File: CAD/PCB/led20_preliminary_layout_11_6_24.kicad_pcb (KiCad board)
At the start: 2 copper layers, 55 x 55 mm, 33 parts, among them U3 Battery, U6 JST

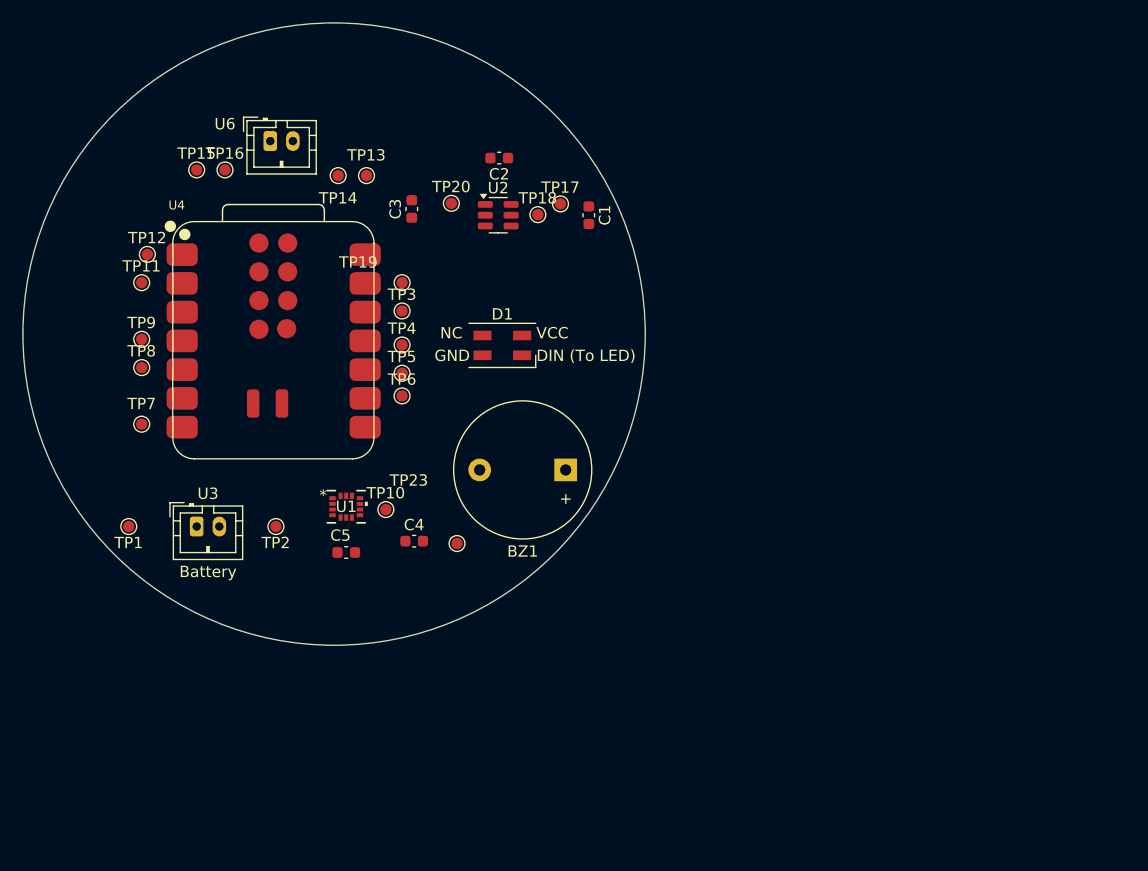
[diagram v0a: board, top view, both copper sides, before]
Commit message: Resubmit
see previous notes
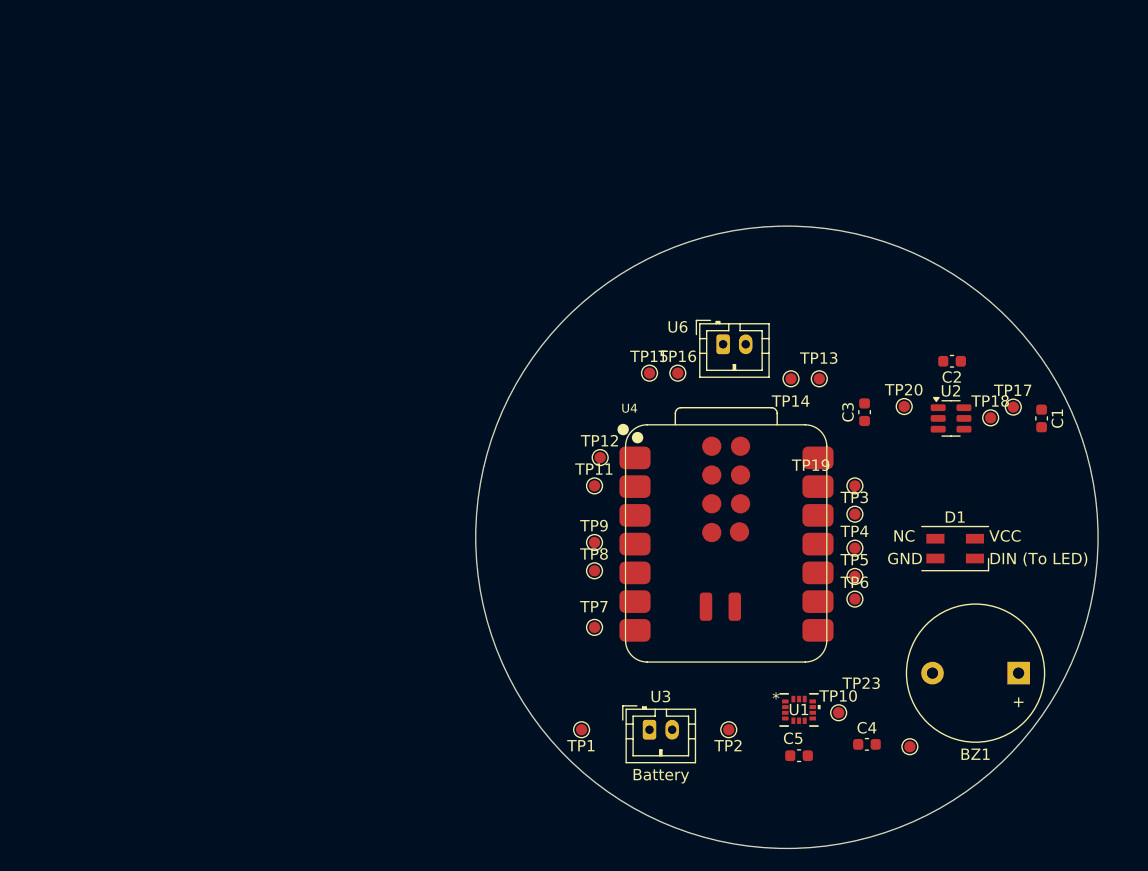
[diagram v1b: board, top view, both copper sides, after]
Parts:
- moved BZ1 43.8 mm to (163.6, 90.0)
- moved C2 43.8 mm to (157.7, 62.5)
- moved C3 43.8 mm to (150.0, 67.0)
- moved D1 43.8 mm to (158.0, 79.0)
- moved TP1 43.8 mm to (125.0, 95.0)
- moved TP11 43.8 mm to (126.1, 73.5)
- moved TP12 43.8 mm to (126.6, 71.0)
- moved TP13 43.8 mm to (146.0, 64.0)
- moved TP14 43.8 mm to (143.5, 64.0)
- moved TP15 43.8 mm to (131.0, 63.5)
- moved TP16 43.8 mm to (133.5, 63.5)
- moved TP2 43.8 mm to (138.0, 95.0)
- moved TP20 43.8 mm to (153.5, 66.5)
- moved TP23 43.8 mm to (154.0, 96.5)
- moved TP7 43.8 mm to (126.1, 86.0)
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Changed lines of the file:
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@@
 		(legacy_teardrops no)
 	)
-	(paper "A5")
+	(paper "A4")
 	(title_block
 		(title "LED20 Preliminary PCB Layout")
@@
 		(allow_soldermask_bridges_in_footprints no)
 		(pcbplotparams
-			(layerselection 0x0001000_7ffffffe)
+			(layerselection 0x0040000_7ffffffe)
 			(plot_on_all_layers_selection 0x7ffffff_80000001)
 			(disableapertmacros no)
@@
 			(drillshape 0)
 			(scaleselection 1)
-			(outputdirectory "./")
+			(outputdirectory "")
 		)
 	)
@@
 	(footprint "Connector_JST:JST_PH_B2B-PH-K_1x02_P2.00mm_Vertical"
 		(layer "F.Cu")
-		(at 97.5 43)
+		(at 137.5 60.95)
 		(descr "JST PH series connector, B2B-PH-K (http://www.jst-mfg.com/product/pdf/eng/ePH.pdf), generated with kicad-footprint-generator")
 		(tags "connector JST PH side entry")
@@
 	(footprint "TestPoint:TestPoint_Pad_D1.0mm"
 		(layer "F.Cu")
-		(at 98 77.05 180)
+		(at 138 95 180)
 		(descr "SMD pad as test Point, diameter 1.0mm")
 		(tags "test point SMD pad")
@@
 	(footprint "Led20:ChargePump"
 		(layer "F.Cu")
-		(at 117.6375 49.55)
+		(at 157.6375 67.5)
 		(descr "SOT, 6 Pin (~), generated with kicad-footprint-generator ipc_gullwing_generator.py")
 		(tags "SOT TO_SOT_SMD")
@@
 	(footprint "TestPoint:TestPoint_Pad_D1.0mm"
 		(layer "F.Cu")
-		(at 107.7103 75.549999)
+		(at 147.7103 93.499999)
 		(descr "SMD pad as test Point, diameter 1.0mm")
 		(tags "test point SMD pad")
@@
 	(footprint "TestPoint:TestPoint_Pad_D1.0mm"
 		(layer "F.Cu")
-		(at 114 78.55)
+		(at 154 96.5)
 		(descr "SMD pad as test Point, diameter 1.0mm")
 		(tags "test point SMD pad")
@@
 	(footprint "LED_SMD:LED_SK6812MINI_PLCC4_3.5x3.5mm_P1.75mm"
 		(layer "F.Cu")
-		(at 118 61.05)
+		(at 158 79)
 		(descr "3.5mm x 3.5mm PLCC4 Addressable RGB LED NeoPixel, https://cdn-shop.adafruit.com/product-files/2686/SK6812MINI_REV.01-1-2.pdf")
 		(tags "LED RGB NeoPixel Mini PLCC-4 3535")
@@
 	(footprint "Capacitor_SMD:C_0603_1608Metric"
 		(layer "F.Cu")
-		(at 110 49 90)
+		(at 150 66.95 90)
 		(descr "Capacitor SMD 0603 (1608 Metric), square (rectangular) end terminal, IPC_7351 nominal, (Body size source: IPC-SM-782 page 76, https://www.pcb-3d.com/wordpress/wp-content/uploads/ipc-sm-782a_amendment_1_and_2.pdf), generated with kicad-footprint-generator")
 		(tags "capacitor")
@@
 	(footprint "TestPoint:TestPoint_Pad_D1.0mm"
 		(layer "F.Cu")
-		(at 86.1444 63.01)
+		(at 126.1444 80.96)
 		(descr "SMD pad as test Point, diameter 1.0mm")
 		(tags "test point SMD pad")
@@
 	(footprint "TestPoint:TestPoint_Pad_D1.0mm"
 		(layer "F.Cu")
-		(at 91 45.55)
+		(at 131 63.5)
 		(descr "SMD pad as test Point, diameter 1.0mm")
 		(tags "test point SMD pad")
@@
 	(footprint "Connector_JST:JST_PH_B2B-PH-K_1x02_P2.00mm_Vertical"
 		(layer "F.Cu")
-		(at 91 77.05)
+		(at 131 95)
 		(descr "JST PH series connector, B2B-PH-K (http://www.jst-mfg.com/product/pdf/eng/ePH.pdf), generated with kicad-footprint-generator")
 		(tags "connector JST PH side entry")
@@
 	(footprint "TestPoint:TestPoint_Pad_D1.0mm"
 		(layer "F.Cu")
-		(at 93.5 45.55)
+		(at 133.5 63.5)
 		(descr "SMD pad as test Point, diameter 1.0mm")
 		(tags "test point SMD pad")
@@
 	(footprint "Capacitor_SMD:C_0603_1608Metric"
 		(layer "F.Cu")
-		(at 104.2103 79.343699)
+		(at 144.2103 97.293699)
 		(descr "Capacitor SMD 0603 (1608 Metric), square (rectangular) end terminal, IPC_7351 nominal, (Body size source: IPC-SM-782 page 76, https://www.pcb-3d.com/wordpress/wp-content/uploads/ipc-sm-782a_amendment_1_and_2.pdf), generated with kicad-footprint-generator")
 		(tags "capacitor")
@@
 	(footprint "Led20:LGA-14L_2P5X3X0P83_STM-L"
 		(layer "F.Cu")
-		(at 104.2103 75.299999)
+		(at 144.2103 93.249999)
 		(tags "LSM6DSO32TR ")
 		(property "Reference" "U1"
@@
 	(footprint "TestPoint:TestPoint_Pad_D1.0mm"
 		(layer "F.Cu")
-		(at 86.1444 68.01)
+		(at 126.1444 85.96)
 		(descr "SMD pad as test Point, diameter 1.0mm")
 		(tags "test point SMD pad")
@@
 	(footprint "Led20:XIAO-ESP32-C6-SMD"
 		(layer "F.Cu")
-		(at 98 60.63)
+		(at 138 78.58)
 		(property "Reference" "U4"
 			(at -9.5 -11.5 0)
@@
 	(footprint "TestPoint:TestPoint_Pad_D1.0mm"
 		(layer "F.Cu")
-		(at 106 46.05)
+		(at 146 64)
 		(descr "SMD pad as test Point, diameter 1.0mm")
 		(tags "test point SMD pad")
@@
 	(footprint "TestPoint:TestPoint_Pad_D1.0mm"
 		(layer "F.Cu")
-		(at 121.1375 49.5)
+		(at 161.1375 67.45)
 		(descr "SMD pad as test Point, diameter 1.0mm")
 		(tags "test point SMD pad")
@@
 	(footprint "Capacitor_SMD:C_0603_1608Metric"
 		(layer "F.Cu")
-		(at 125.6375 49.55 -90)
+		(at 165.6375 67.5 -90)
 		(descr "Capacitor SMD 0603 (1608 Metric), square (rectangular) end terminal, IPC_7351 nominal, (Body size source: IPC-SM-782 page 76, https://www.pcb-3d.com/wordpress/wp-content/uploads/ipc-sm-782a_amendment_1_and_2.pdf), generated with kicad-footprint-generator")
 		(tags "capacitor")
@@
 	(footprint "Buzzer_Beeper:Buzzer_12x9.5RM7.6"
 		(layer "F.Cu")
-		(at 123.6 72.05 180)
+		(at 163.6 90 180)
 		(descr "Generic Buzzer, D12mm height 9.5mm with RM7.6mm")
 		(tags "buzzer")
@@
 	(footprint "TestPoint:TestPoint_Pad_D1.0mm"
 		(layer "F.Cu")
-		(at 103.5 46.05)
+		(at 143.5 64)
 		(descr "SMD pad as test Point, diameter 1.0mm")
 		(tags "test point SMD pad")
@@
 	(footprint "TestPoint:TestPoint_Pad_D1.0mm"
 		(layer "F.Cu")
-		(at 85 77.05 180)
+		(at 125 95 180)
 		(descr "SMD pad as test Point, diameter 1.0mm")
 		(tags "test point SMD pad")
@@
 	(footprint "Capacitor_SMD:C_0603_1608Metric"
 		(layer "F.Cu")
-		(at 117.725 44.5 180)
+		(at 157.725 62.45 180)
 		(descr "Capacitor SMD 0603 (1608 Metric), square (rectangular) end terminal, IPC_7351 nominal, (Body size source: IPC-SM-782 page 76, https://www.pcb-3d.com/wordpress/wp-content/uploads/ipc-sm-782a_amendment_1_and_2.pdf), generated with kicad-footprint-generator")
 		(tags "capacitor")
@@
 	(footprint "TestPoint:TestPoint_Pad_D1.0mm"
 		(layer "F.Cu")
-		(at 123.1375 48.55)
+		(at 163.1375 66.5)
 		(descr "SMD pad as test Point, diameter 1.0mm")
 		(tags "test point SMD pad")
@@
 	(footprint "TestPoint:TestPoint_Pad_D1.0mm"
 		(layer "F.Cu")
-		(at 109.1444 61.01)
+		(at 149.1444 78.96)
 		(descr "SMD pad as test Point, diameter 1.0mm")
 		(tags "test point SMD pad")
@@
 	(footprint "TestPoint:TestPoint_Pad_D1.0mm"
 		(layer "F.Cu")
-		(at 113.5 48.5)
+		(at 153.5 66.45)
 		(descr "SMD pad as test Point, diameter 1.0mm")
 		(tags "test point SMD pad")
@@
 	(footprint "TestPoint:TestPoint_Pad_D1.0mm"
 		(layer "F.Cu")
-		(at 109.1444 58.01)
+		(at 149.1444 75.96)
 		(descr "SMD pad as test Point, diameter 1.0mm")
 		(tags "test point SMD pad")
@@
 	(footprint "TestPoint:TestPoint_Pad_D1.0mm"
 		(layer "F.Cu")
-		(at 109.1444 55.51)
+		(at 149.1444 73.46)
 		(descr "SMD pad as test Point, diameter 1.0mm")
 		(tags "test point SMD pad")
@@
 	(footprint "TestPoint:TestPoint_Pad_D1.0mm"
 		(layer "F.Cu")
-		(at 109.1444 65.51)
+		(at 149.1444 83.46)
 		(descr "SMD pad as test Point, diameter 1.0mm")
 		(tags "test point SMD pad")
@@
 	(footprint "TestPoint:TestPoint_Pad_D1.0mm"
 		(layer "F.Cu")
-		(at 86.6444 53.01)
+		(at 126.6444 70.96)
 		(descr "SMD pad as test Point, diameter 1.0mm")
 		(tags "test point SMD pad")
@@
 	(footprint "TestPoint:TestPoint_Pad_D1.0mm"
 		(layer "F.Cu")
-		(at 86.1444 55.51)
+		(at 126.1444 73.46)
 		(descr "SMD pad as test Point, diameter 1.0mm")
 		(tags "test point SMD pad")
@@
 	(footprint "TestPoint:TestPoint_Pad_D1.0mm"
 		(layer "F.Cu")
-		(at 109.1444 63.51)
+		(at 149.1444 81.46)
 		(descr "SMD pad as test Point, diameter 1.0mm")
 		(tags "test point SMD pad")
@@
 	(footprint "TestPoint:TestPoint_Pad_D1.0mm"
 		(layer "F.Cu")
-		(at 86.1444 60.51)
+		(at 126.1444 78.46)
 		(descr "SMD pad as test Point, diameter 1.0mm")
 		(tags "test point SMD pad")
@@
 	(footprint "Capacitor_SMD:C_0603_1608Metric"
 		(layer "F.Cu")
-		(at 110.2103 78.343699)
+		(at 150.2103 96.293699)
 		(descr "Capacitor SMD 0603 (1608 Metric), square (rectangular) end terminal, IPC_7351 nominal, (Body size source: IPC-SM-782 page 76, https://www.pcb-3d.com/wordpress/wp-content/uploads/ipc-sm-782a_amendment_1_and_2.pdf), generated with kicad-footprint-generator")
 		(tags "capacitor")
@@
 	)
 	(gr_circle
-		(center 103.1375 60.05)
-		(end 123 41.05)
+		(center 143.1375 78)
+		(end 163 59)
 		(stroke
 			(width 0.05)
@@
 	)
 	(gr_text "NC"
-		(at 112.5 60.55 0)
+		(at 152.5 78.5 0)
 		(layer "F.SilkS")
 		(effects
@@
 	)
 	(gr_text "DIN (To LED)\n"
-		(at 121 62.55 0)
+		(at 161 80.5 0)
 		(layer "F.SilkS")
 		(effects
@@
 	)
 	(gr_text "GND\n"
-		(at 112 62.55 0)
+		(at 152 80.5 0)
 		(layer "F.SilkS")
 		(effects
@@
 	)
 	(gr_text "VCC"
-		(at 121 60.55 0)
+		(at 161 78.5 0)
 		(layer "F.SilkS")
 		(effects
